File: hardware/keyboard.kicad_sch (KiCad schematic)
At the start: 41 parts, among them SW1 SW_Push, SW10 SW_Push, SW11 SW_Push, SW12 SW_Push, SW13 SW_Push, SW14 SW_Push, SW15 SW_Push, SW16 SW_Push, SW17 SW_Push, SW18 SW_Push, SW19 SW_Push, SW2 SW_Push, SW20 SW_Push, SW21 SW_Push, SW22 SW_Push, SW23 SW_Push, SW24 SW_Push, SW25 SW_Push, SW26 SW_Push, SW27 SW_Push, SW28 SW_Push, SW29 SW_Push, SW3 SW_Push, SW30 SW_Push, SW31 SW_Push, SW32 SW_Push, SW33 SW_Push, SW34 SW_Push, SW35 SW_Push, SW36 SW_Push, SW37 SW_Push, SW38 SW_Push, SW39 SW_Push, SW4 SW_Push, SW40 SW_Push, SW5 SW_Push, SW6 SW_Push, SW7 SW_Push, SW8 SW_Push, SW9 SW_Push, U2 74HC138

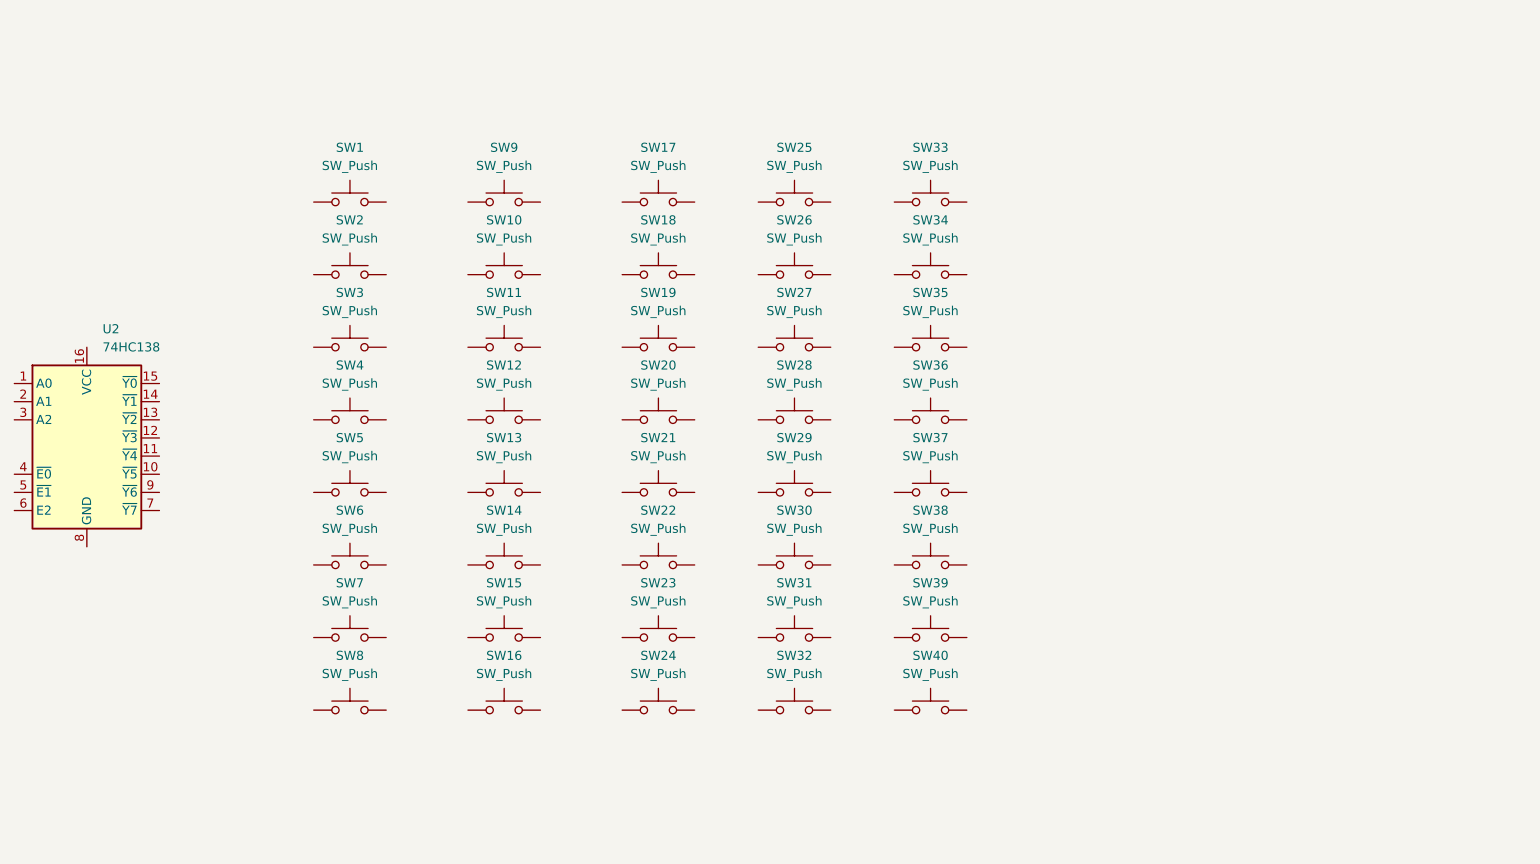
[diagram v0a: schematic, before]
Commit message: keyboard schematic
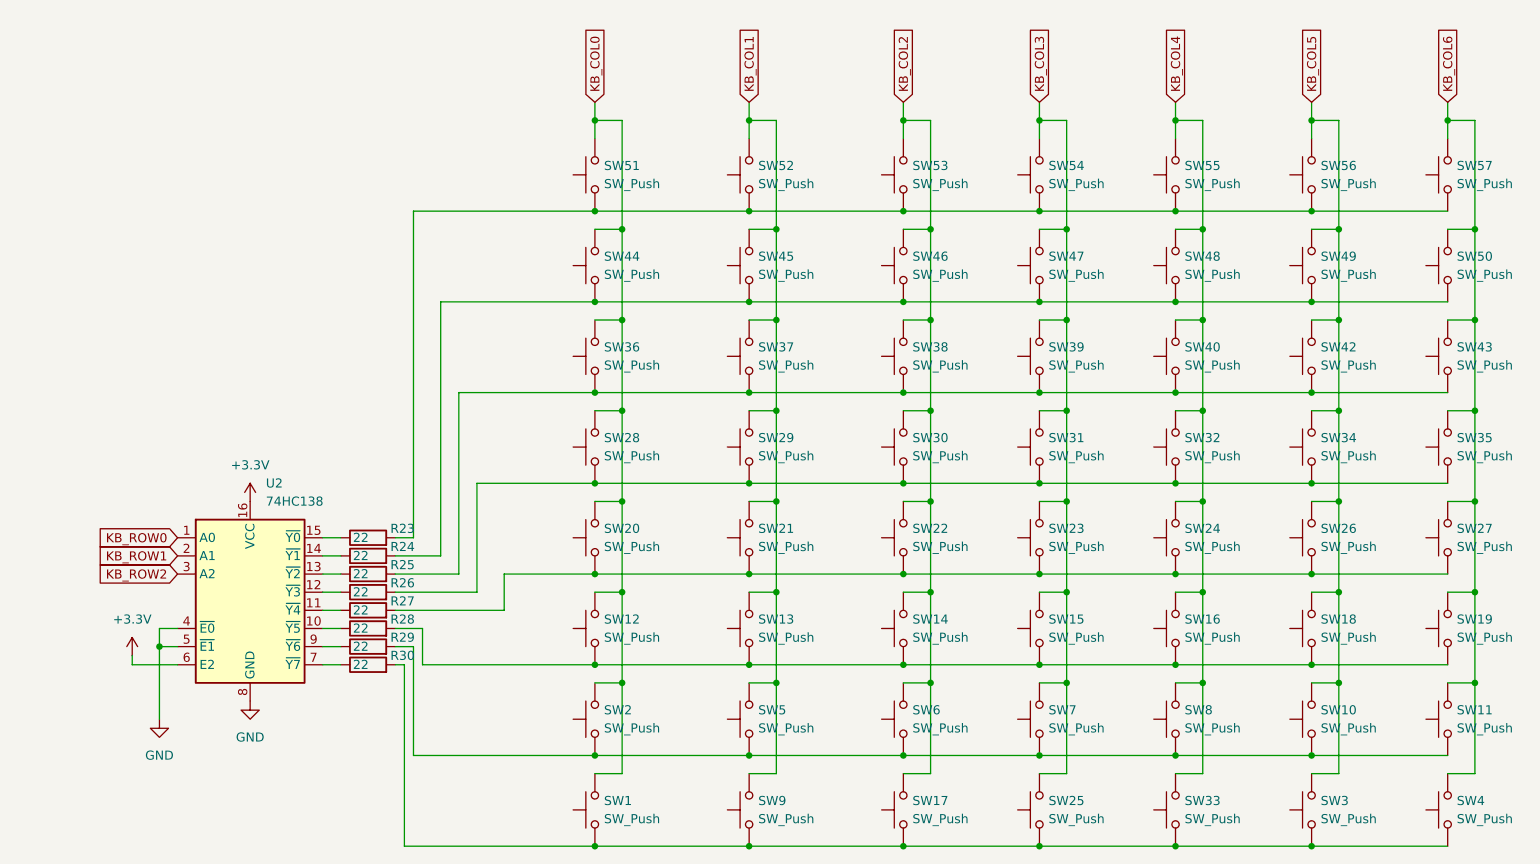
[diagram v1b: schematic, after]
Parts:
- added R23, R24, R25, R26, R27, R28, R29, R30: 22, symbol Device:R
- added SW42, SW43, SW44, SW45, SW46, SW47, SW48, SW49, SW50, SW51, SW52, SW53, SW54, SW55, SW56, SW57: SW_Push, Button_Switch_SMD:SW_Push_1P1T_NO_6x6mm_H9.5mm, symbol Switch:SW_Push
- U2: LCSC (none) -> C2906780
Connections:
- net at SW34.1: now also SW28.1, SW29.1, SW30.1, SW31.1, SW32.1, SW35.1, R26.2
- net KB_COL5: now reaches SW34.2
- net KB_COL5: now also SW10.2, SW18.2, SW26.2, SW3.2, SW42.2, SW49.2, SW56.2
- net at SW14.1: now also SW12.1, SW13.1, SW15.1, SW16.1, SW18.1, SW19.1, R28.2
- net KB_COL2: now reaches SW14.2
- net KB_COL2: now also SW17.2, SW22.2, SW30.2, SW38.2, SW6.2, SW46.2, SW53.2
- net at SW33.1: now also SW1.1, SW17.1, SW25.1, SW3.1, SW4.1, SW9.1, R30.2
- net KB_COL4: now reaches SW33.2
- net KB_COL4: now also SW16.2, SW24.2, SW32.2, SW40.2, SW8.2, SW48.2, SW55.2
- net at SW6.1: now also SW10.1, SW11.1, SW2.1, SW5.1, SW7.1, SW8.1, R29.2
- net KB_COL3: now reaches SW31.2
- net KB_COL3: now also SW15.2, SW23.2, SW25.2, SW39.2, SW7.2, SW47.2, SW54.2
- net KB_COL1: now reaches SW9.2
- net KB_COL1: now also SW13.2, SW21.2, SW29.2, SW37.2, SW5.2, SW45.2, SW52.2
- net KB_COL6: now reaches SW11.2
- net KB_COL6: now also SW19.2, SW27.2, SW35.2, SW4.2, SW43.2, SW50.2, SW57.2
- net at SW39.1: now also SW36.1, SW37.1, SW38.1, SW40.1, R25.2, SW42.1, SW43.1
- net KB_COL0: now reaches SW1.2
- net KB_COL0: now also SW12.2, SW2.2, SW20.2, SW28.2, SW36.2, SW44.2, SW51.2
- net at SW23.1: now also SW20.1, SW21.1, SW22.1, SW24.1, SW26.1, SW27.1, R27.2
- net KB_ROW0: now reaches U2.1 (A0)
- net at U2.10 (~{Y5}): now also R28.1
- net at U2.11 (~{Y4}): now also R27.1
- net at U2.12 (~{Y3}): now also R26.1
- net at U2.13 (~{Y2}): now also R25.1
- net at U2.14 (~{Y1}): now also R24.1
- net at U2.15 (~{Y0}): now also R23.1
- net +3.3V: now reaches U2.16 (VCC)
- net +3.3V: now also U2.6 (E2)
- net KB_ROW1: now reaches U2.2 (A1)
- net KB_ROW2: now reaches U2.3 (A2)
- net GND: now reaches U2.4 (~{E0})
- net GND: now also U2.5 (~{E1}), U2.8 (GND)
- net at U2.7 (~{Y7}): now also R30.1
- net at U2.9 (~{Y6}): now also R29.1
- new net: R24.2, SW44.1, SW45.1, SW46.1, SW47.1, SW48.1, SW49.1, SW50.1
- new net: R23.2, SW51.1, SW52.1, SW53.1, SW54.1, SW55.1, SW56.1, SW57.1
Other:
- moved on the sheet: SW1, SW17, SW25, SW33, SW9, U2
